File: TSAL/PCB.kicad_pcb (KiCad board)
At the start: 4 copper layers, 100 x 100 mm, 74 parts, among them J1 TE 770966-2, J2 JST B04B-XASK, J3 TE 770966-2, J4 TE 770966-2, Q1 IRLZ44N, Q2 MMBT3904, Q3 IRLZ44N, Q4 STD7NK40Z, T1 11328-T078, U1 TL431D, U2 LMV331, U3 VRB1205YMD-15WR3, U4 LTV-817S, U5 LM555xN, U6 LT8316IFE#PBF

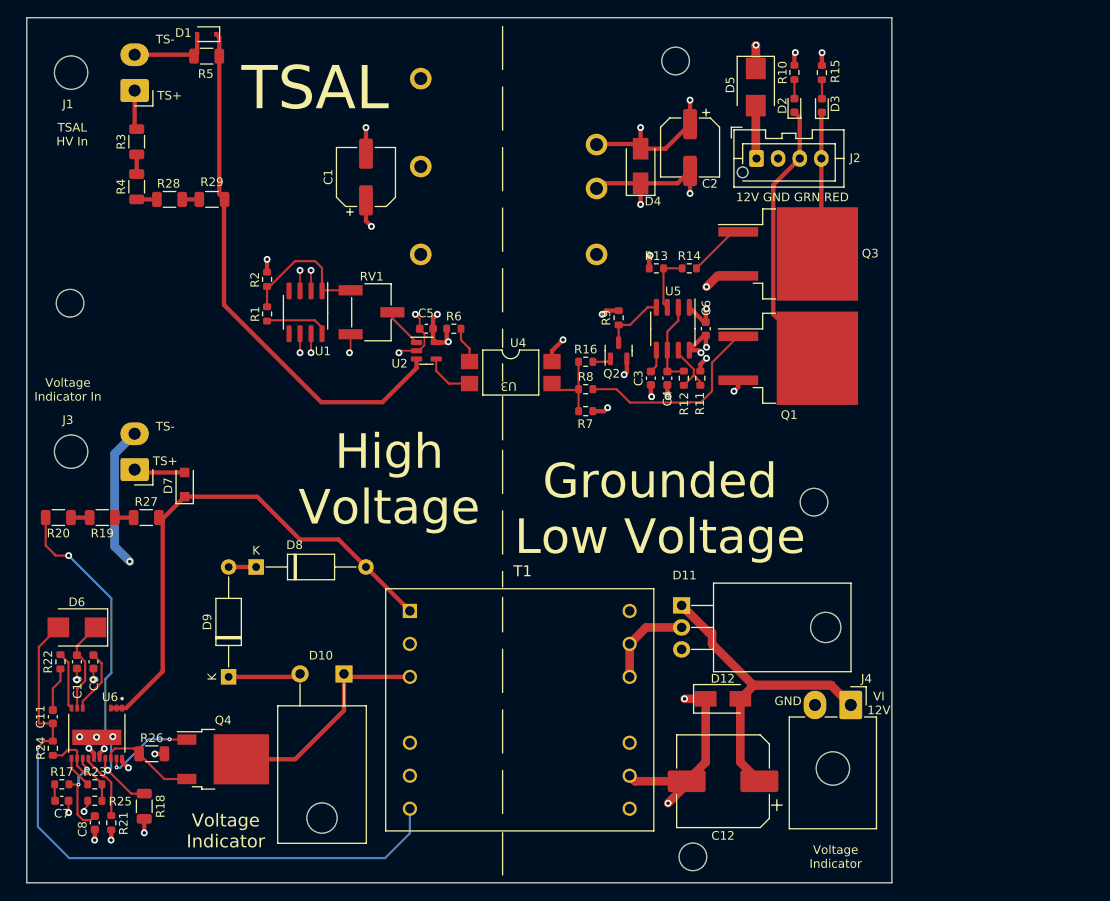
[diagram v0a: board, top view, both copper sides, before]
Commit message: TSAL V2
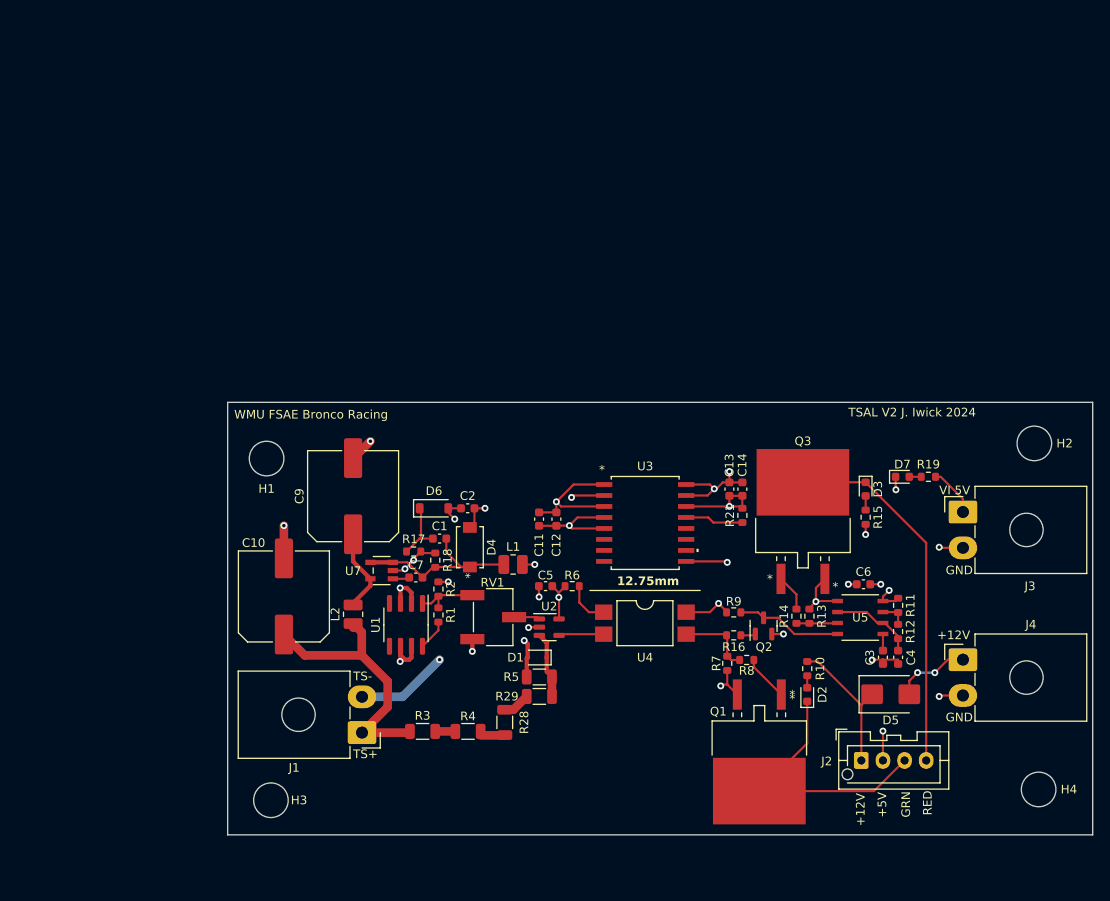
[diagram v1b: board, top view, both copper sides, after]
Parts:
- removed C8: 47p, Capacitor_SMD:C_0603_1608Metric
- removed D10: RFN5TF8S, Package_TO_SOT_THT:TO-220-2_Horizontal_TabDown
- removed D11: RB238T150, Package_TO_SOT_THT:TO-220-3_Horizontal_TabDown
- removed D12: SMAJ15CA, Diode_SMD:D_SMA
- removed D8, D9: 1N5375B, Diode_THT:D_A-405_P12.70mm_Horizontal
- removed Q4: STD7NK40Z, Package_TO_SOT_SMD:TO-252-2
- removed R20, R27: 500k, Resistor_SMD:R_1206_3216Metric
- removed R22: 10k, Resistor_SMD:R_0603_1608Metric
- removed R23: 121k, Resistor_SMD:R_0603_1608Metric
- removed R24: 44.2k, Resistor_SMD:R_0603_1608Metric
- removed R25: 4.99k, Resistor_SMD:R_0603_1608Metric
- removed R26: 0.05, Resistor_SMD:R_1206_3216Metric
- removed T1: 11328-T078, 11328-T078:11328T078
- removed U6: LT8316IFE#PBF, kicad-libraries:IC_LT8316IFE#PBF
- added C13: 10u, Capacitor_SMD:C_0603_1608Metric, F.Cu at (160.2, 96.5)
- added C14: 0.1u, Capacitor_SMD:C_0603_1608Metric, F.Cu at (161.8, 96.5)
- added L1: 1.2m, Inductor_SMD:L_1008_2520Metric, F.Cu at (135.2, 105.2)
- added L2: 1m, Inductor_SMD:L_1008_2520Metric, F.Cu at (116.8, 111.0)
- added U7: MP174AGJ-Z, MP174AGJ_Z:TSOT23-5_MP174A_MNP, F.Cu at (120.0, 106.0)
- C1: value 100u -> 100n; footprint Capacitor_SMD:CP_Elec_6.3x7.7 -> Capacitor_SMD:C_0603_1608Metric
- C10, C9: value 4.7u -> 500V 3.9u; footprint Capacitor_SMD:C_0603_1608Metric -> Capacitor_SMD:C_Elec_10x10.2
- C11: value 47p -> 10u
- C12: value 470uF -> 0.1u; footprint Capacitor_SMD:CP_Elec_10x10.5 -> Capacitor_SMD:C_0603_1608Metric
- C2: footprint Capacitor_SMD:CP_Elec_6.3x7.7 -> Capacitor_SMD:C_0603_1608Metric
- C3, C5, C6: value 100nF -> 100n
- C7: value 100nF -> 2.2u
- D4: value SMAJ15CA -> AES2JF-HF; footprint Diode_SMD:D_SMA -> KiCADv6:CR_SMAF_CIP
- D6: value SK520B -> 1N4007; footprint Diode_SMD:D_SMB -> Diode_SMD:D_SOD-123
- D7: value 1N4007FL -> LED-Red; footprint Diode_SMD:D_SOD-123F -> LED_SMD:LED_0603_1608Metric
- H1, H2, H3, H4: value MountingHole_3.2mm_M3_ISO14580 -> MountingHole; footprint MountingHole:MountingHole_3.2mm_M3_ISO14580 -> MountingHole:MountingHole_4mm
- J3, J4: value TE 770966-2 -> Conn_01x02
- Q1, Q3: footprint Package_TO_SOT_SMD:TO-263-2 -> IRLZ44NSTRLPBF:NMOSGDS_D2PAK_INF
- R15: value 2.2k -> 1k
- R17: value 10k -> 5k
- R18: value 40k -> 5k; footprint Resistor_SMD:R_1206_3216Metric -> Resistor_SMD:R_0603_1608Metric
- R19: value 500k -> 1k; footprint Resistor_SMD:R_1206_3216Metric -> Resistor_SMD:R_0603_1608Metric
- R21: value 56.2k -> 0
- U3: value VRB1205YMD-15WR3 -> UCC12040DVE; footprint VRB1205YMD-6WR3:VRB1205YMD-15WR3 -> footprints:SO_0DVER_TEX
- U5: footprint Package_SO:SOIC-8_3.9x4.9mm_P1.27mm -> footprints 555:M08A-L
- moved J3 95.9 mm to (187.2, 99.2), turned to 0 degrees
- moved R19 95.6 mm to (183.2, 95.1), turned to 0 degrees
- moved D7 83.0 mm to (180.2, 95.1), turned to 0 degrees
- moved D1 81.6 mm to (138.0, 116.0)
- moved R5 81.4 mm to (138.3, 118.2)
- moved R21 81.1 mm to (161.8, 99.6), turned to 90 degrees
- moved J1 78.7 mm to (117.8, 124.7)
- moved R3 75.8 mm to (124.8, 124.5), turned to 0 degrees
- moved R4 73.7 mm to (130.0, 124.5), turned to 0 degrees
- moved D5 71.9 mm to (178.9, 120.2), turned to 0 degrees
- moved R28 71.8 mm to (134.3, 123.5), turned to 90 degrees
- moved H3 71.6 mm to (107.2, 132.5)
- moved J2 70.6 mm to (175.5, 127.9)
- moved G*** 70.6 mm to (150.2, 116.2)
- moved R10 68.9 mm to (169.2, 117.3)
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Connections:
- C1 pad 1: +5V -> Net-(D6-K)
- C1 pad 2: TS- -> Net-(D4-K)
- C10 pad 1: VI- -> TS+
- C10 pad 2: Net-(C10-Pad2) -> TS-
- C11 pad 1: Net-(C11-Pad1) -> +5V
- C11 pad 2: Net-(C11-Pad2) -> TS-
- C12 pad 1: Net-(C12-Pad1) -> +5V
- C12 pad 2: GND -> TS-
- C2 pad 1: +12V -> +5V
- C2 pad 2: GND -> TS-
- C4 pad 1: Net-(C4-Pad1) -> GND
- C4 pad 2: GND -> Net-(U5-THR)
- C6 pad 1: +12V -> +5V@GLV
- C7 pad 1: Net-(C7-Pad1) -> Net-(U7-VCC)
- C7 pad 2: VI- -> Net-(D4-K)
- C9 pad 1: VI- -> Net-(U7-DRAIN)
- C9 pad 2: Net-(C9-Pad2) -> TS-
- D4 pad 1: GND -> Net-(D4-K)
- D4 pad 2: +12V -> TS-
- D5 pad 2: Net-(D5-Pad2) -> Net-(D5-A)
- D6 pad 1: Net-(C10-Pad2) -> Net-(D6-K)
- D6 pad 2: Net-(C11-Pad1) -> +5V
- D7 pad 1: VI+ -> GND
- D7 pad 2: Net-(D7-Pad2) -> Net-(D7-A)
- J2 pad 1: Net-(D5-Pad2) -> +12V
- J2 pad 2: GND -> +5V@GLV
- J3 pad 1: Net-(D7-Pad2) -> +5V@GLV
- J3 pad 2: VI- -> GND
- J4 pad 1: Net-(C12-Pad1) -> Net-(D5-A)
- R11 pad 1: +12V -> +5V@GLV
- R12 pad 2: Net-(C4-Pad1) -> Net-(U5-THR)
- R15 pad 2: +12V -> +5V@GLV
- R17 pad 1: Net-(C7-Pad1) -> Net-(D6-K)
- R17 pad 2: Net-(C8-Pad1) -> Net-(U7-FB)
- R18 pad 1: VI- -> Net-(U7-FB)
- R18 pad 2: Net-(R18-Pad2) -> Net-(D4-K)
- R19 pad 1: Net-(R19-Pad1) -> Net-(D7-A)
- R19 pad 2: Net-(R19-Pad2) -> +5V@GLV
- R21 pad 1: Net-(R21-Pad1) -> Net-(U3-SEL)
- R21 pad 2: VI- -> +5V@GLV
- R9 pad 2: +12V -> +5V@GLV
- U3 pad 1: +12V -> +5V
- U3 pad 2: GND -> TS-
- U3 pad 3: +12V -> +5V
- U3 pad 4: +5V -> TS-
- U3 pad 5: unconnected-(U3-Pad5) -> TS-
- U3 pad 6: TS- -> unconnected-(U3-NC-Pad6)
- U4 pad 4: +12V -> +5V@GLV
- U5 pad 2: Net-(C4-Pad1) -> Net-(U5-THR)
- U5 pad 6: Net-(C4-Pad1) -> Net-(U5-THR)
- U5 pad 8: +12V -> +5V@GLV
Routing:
- net Net-(C11-Pad1): track 75.4 -> 0.00 mm, vias 1 -> 0
- net VI+: track 61.2 -> 0.00 mm
- net Net-(D1-K): track 61.3 -> 7.66 mm
- net Net-(C12-Pad1): track 46.6 -> 0.00 mm
- net Net-(R18-Pad2): track 40.9 -> 0.00 mm, vias 2 -> 0
- net +5V@GLV: track 0.00 -> 31.7 mm, vias 0 -> 6
- net VI-: track 31.2 -> 0.00 mm, vias 15 -> 0
- net TS+: track 4.56 -> 30.9 mm
- net Net-(D10-Pad1): track 26.2 -> 0.00 mm
- net /Ext-LED-RED: track 16.6 -> 42.3 mm
- net TS-: track 31.3 -> 55.9 mm, vias 8 -> 12
- net Net-(D4-K): track 0.00 -> 21.8 mm
- net +12V: track 35.5 -> 16.5 mm, vias 10 -> 0
- net Net-(Q1-G): track 22.6 -> 5.32 mm
- net GND: track 57.9 -> 40.8 mm, vias 12 -> 11
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- added copper zone on In1.Cu, net +5V@GLV
- added copper zone on In2.Cu, net GND
- removed copper zone on In2.Cu, net +12V
- removed copper zone on In1.Cu, net GND
- removed copper zone on In1.Cu, net VI-
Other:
- board size 100 x 100 mm -> 100 x 50 mm
- board text added: "+12V"
- board text added: "+5V"
- board text added: "12.75mm"
- board text added: "Bronco Racing TSAL + Voltage Indicator Rev 2"
- board text added: "GRN"
- board text added: "RED"
- board text added: "TSAL V2 J. Iwick 2024"
- board text added: "VI 5V"
- board text added: "WMU FSAE Bronco Racing"
- board text removed: "12V GND GRN RED"
- board text removed: "Bronco Racing TSAL + Voltage Indicator Rev 1"
- board text removed: "Grounded Low Voltage"
- board text removed: "High Voltage"
- board text removed: "TSAL"
- board text removed: "TSAL HV In"
- board text removed: "VI 12V"
- board text removed: "Voltage Indicator"
- board text removed: "Voltage Indicator In"
